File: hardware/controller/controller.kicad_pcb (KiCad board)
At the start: 2 copper layers, 1 part

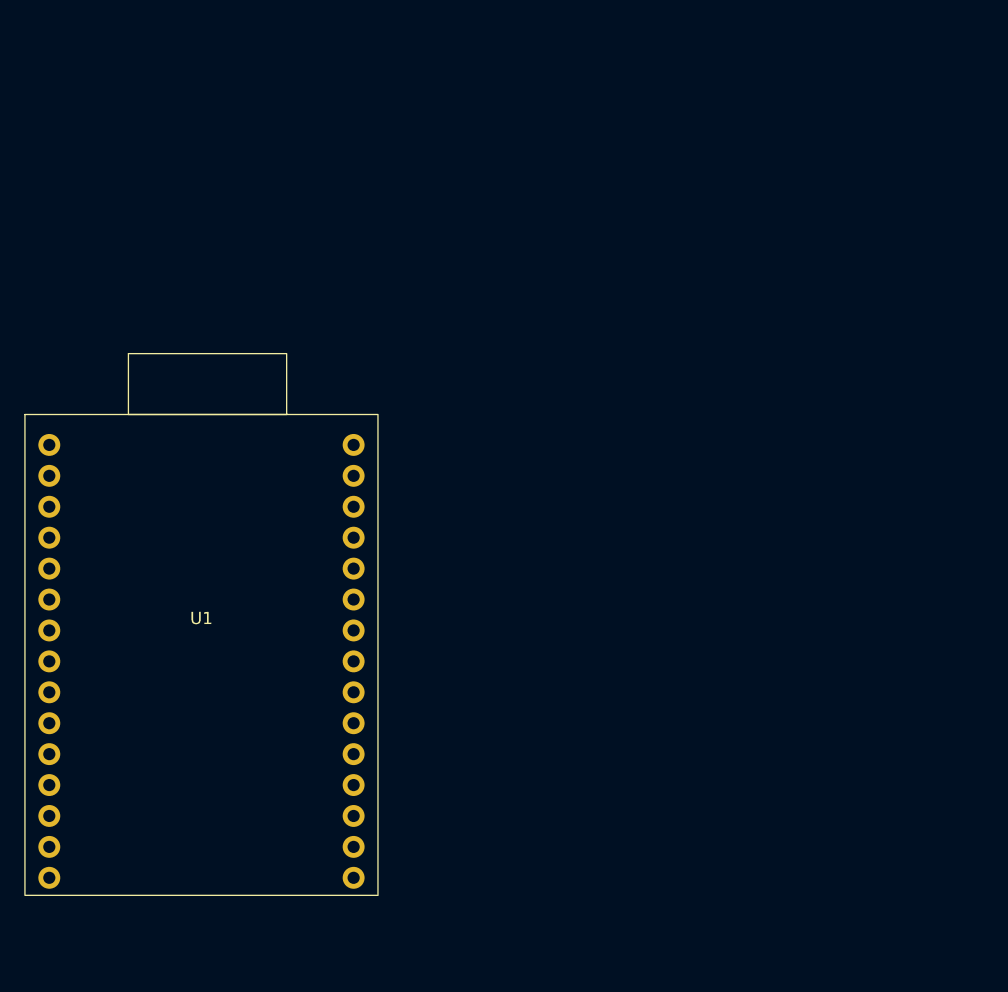
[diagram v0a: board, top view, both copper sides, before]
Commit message: (frature): add pcb controller
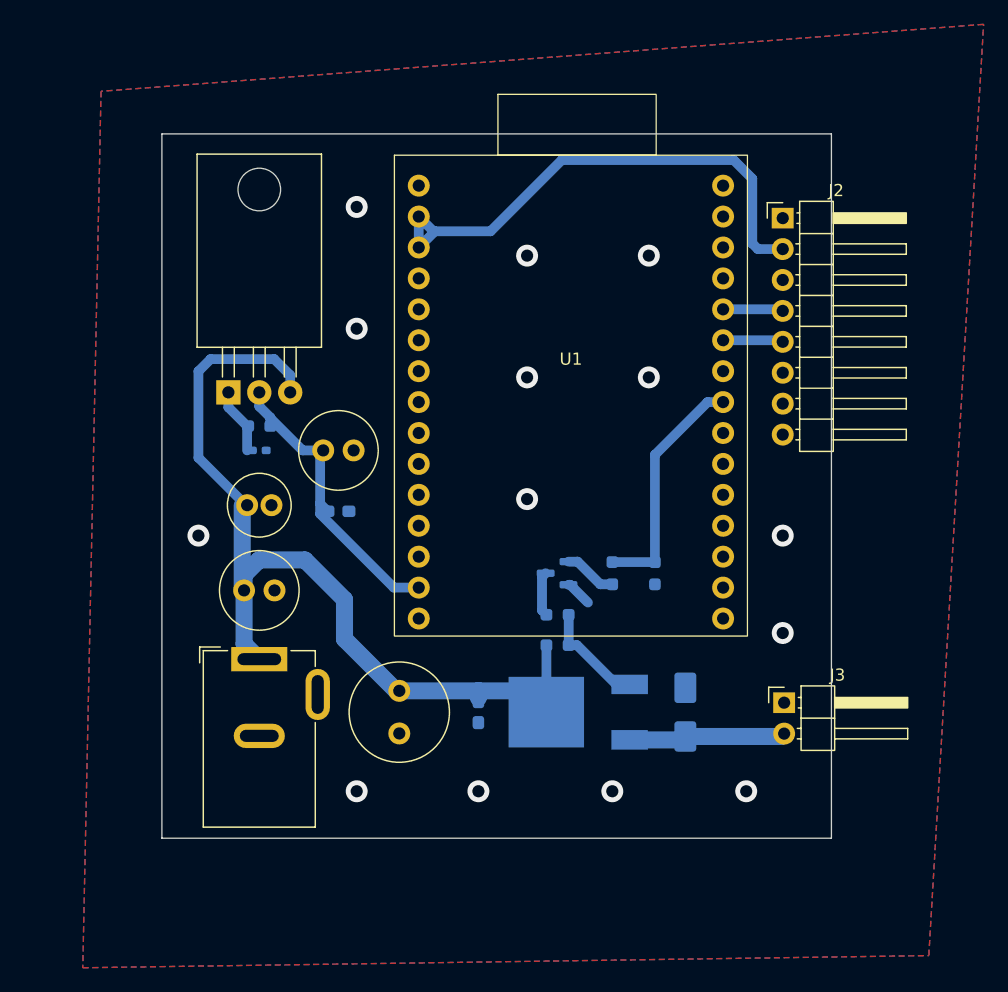
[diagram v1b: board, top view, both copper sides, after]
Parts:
- added C1: 100uF, Capacitor_THT:C_Radial_D6.3mm_H11.0mm_P2.50mm, F.Cu at (126.8, 97.5)
- added C2: 100nF, Capacitor_SMD:C_0603_1608Metric_Pad1.08x0.95mm_HandSolder, B.Cu at (146.0, 107.5)
- added C3: 470uF, Capacitor_THT:C_Radial_D8.0mm_H11.5mm_P3.50mm, F.Cu at (139.5, 105.8)
- added C4: 100uF, Capacitor_THT:C_Radial_D6.3mm_H11.0mm_P2.50mm, F.Cu at (133.2, 86.0)
- added C5: 10uF, Capacitor_THT:C_Radial_D5.0mm_H11.0mm_P2.00mm, F.Cu at (127.0, 90.5)
- added C6: 100nF, Capacitor_SMD:C_0603_1608Metric_Pad1.08x0.95mm_HandSolder, B.Cu at (134.5, 91.0)
- added D1: SS34, Diode_SMD:D_SMA, B.Cu at (163.0, 107.5)
- added J1: Barrel_Jack_Switch, Connector_BarrelJack:BarrelJack_GCT_DCJ200-10-A_Horizontal, F.Cu at (128.0, 103.2)
- added J2: GY-87 conn, Connector_PinHeader_2.54mm:PinHeader_1x08_P2.54mm_Horizontal, F.Cu at (171.0, 66.9)
- added J3: Ventoinha, Connector_PinHeader_2.54mm:PinHeader_1x02_P2.54mm_Horizontal, F.Cu at (171.1, 106.7)
- added Q1: BC846, Package_TO_SOT_SMD:SOT-23, B.Cu at (152.5, 96.1)
- added Q2: AP9565K, EasyEDA:TO-252-2_L6.6-W6.1-P4.57-LS10.1-BR-CW, B.Cu at (155.0, 107.5)
- added R1: 4.7KR, Resistor_SMD:R_0603_1608Metric_Pad0.98x0.95mm_HandSolder, B.Cu at (152.5, 102.0)
- added R2: 100R, Resistor_SMD:R_0603_1608Metric_Pad0.98x0.95mm_HandSolder, B.Cu at (152.5, 99.5)
- added R3: 4.7KR, Resistor_SMD:R_0603_1608Metric_Pad0.98x0.95mm_HandSolder, B.Cu at (157.0, 96.1)
- added R4: 100KR, Resistor_SMD:R_0603_1608Metric_Pad0.98x0.95mm_HandSolder, B.Cu at (160.5, 96.1)
- added R5: 30.9KR, Resistor_SMD:R_0603_1608Metric_Pad0.98x0.95mm_HandSolder, B.Cu at (128.0, 84.0)
- added R6: 22.1KR, Capacitor_SMD:C_0402_1005Metric_Pad0.74x0.62mm_HandSolder, B.Cu at (128.0, 86.0)
- added U3: LM1117T-ADJ, Package_TO_SOT_THT:TO-220-3_Horizontal_TabDown, F.Cu at (125.5, 81.2)
- moved U1 37.1 mm to (139.1, 61.8)
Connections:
- U1 pad 1: unconnected-(U1-GND-Pad1) -> GND
- U1 pad 12: unconnected-(U1-GND-Pad12) -> GND
- U1 pad 14: unconnected-(U1-5V-Pad14) -> 5V
- U1 pad 15: unconnected-(U1-GND-Pad15) -> GND
- U1 pad 16: unconnected-(U1-GND-Pad16) -> GND
- U1 pad 19: unconnected-(U1-GND-Pad19) -> GND
- U1 pad 2: unconnected-(U1-3V3-Pad2) -> 3V3
- U1 pad 23: unconnected-(U1-GPIO7-Pad23) -> /PWM_CONTROL
- U1 pad 24: unconnected-(U1-GND-Pad24) -> GND
- U1 pad 25: unconnected-(U1-RGB_LED/SDA/GPIO8-Pad25) -> /SDA
- U1 pad 26: unconnected-(U1-BOOT/SCL/GPIO9-Pad26) -> /SCL
- U1 pad 27: unconnected-(U1-GND-Pad27) -> GND
- U1 pad 3: unconnected-(U1-3V3-Pad3) -> 3V3
- U1 pad 30: unconnected-(U1-GND-Pad30) -> GND
- U1 pad 6: unconnected-(U1-GND-Pad6) -> GND
- U1 pad 8: unconnected-(U1-GND-Pad8) -> GND
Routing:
- net 12V: track 0.00 -> 75.7 mm
- net 3V3: track 0.00 -> 43.4 mm
- net 5V: track 0.00 -> 25.4 mm
- net /PWM_CONTROL: track 0.00 -> 19.7 mm
- net Net-(D1-K): track 0.00 -> 12.9 mm
- net Net-(Q2-G): track 0.00 -> 8.84 mm
- net Net-(U3-ADJ): track 0.00 -> 5.53 mm
- net /SCL: track 0.00 -> 4.95 mm
- net /SDA: track 0.00 -> 4.95 mm
- net Net-(Q1-B): track 0.00 -> 4.37 mm
- net Net-(Q1-C): track 0.00 -> 3.69 mm
- net GND: track 0.00 -> 2.21 mm, vias 0 -> 14
- added copper zone on B.Cu, net GND
- added copper zone on F.Cu, net GND
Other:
- board outline added: 55 x 57.9 mm
